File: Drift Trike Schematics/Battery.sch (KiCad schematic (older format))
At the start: 121 parts

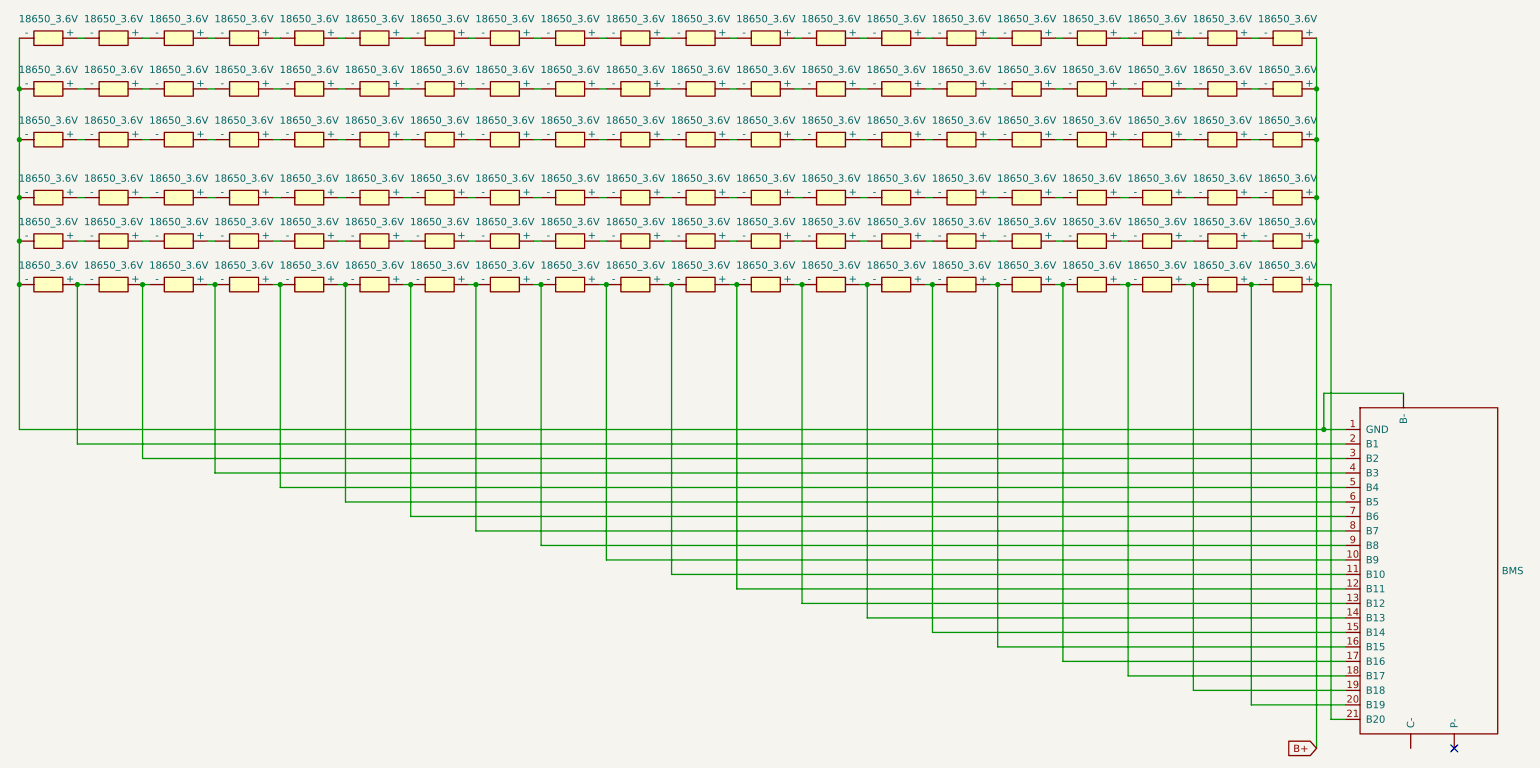
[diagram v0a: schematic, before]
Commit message: Small Fix
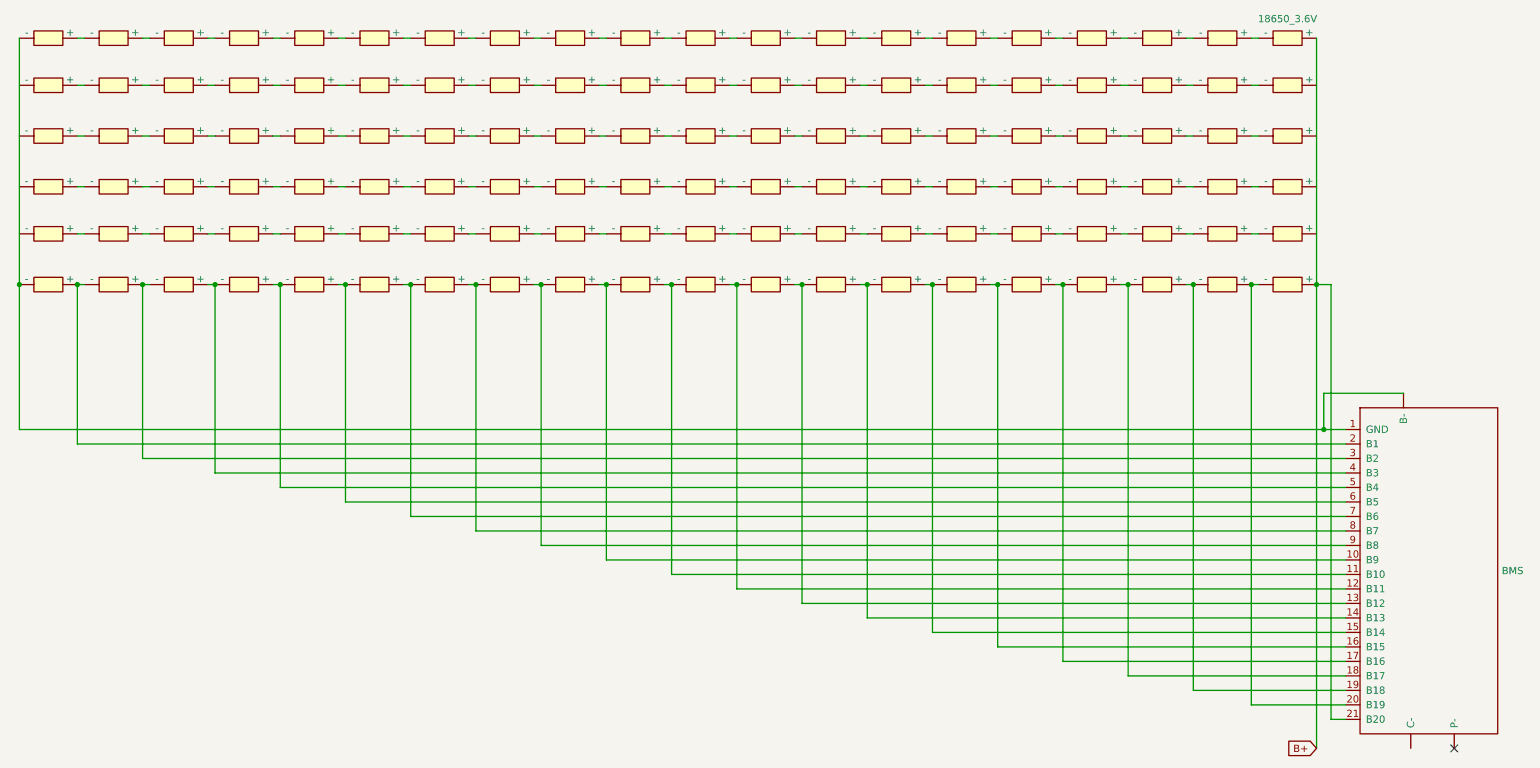
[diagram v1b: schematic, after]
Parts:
- removed U? (x80): 18650_3.6V, symbol trike_lib:18650_3.6V
- added U? (x80): 18650_3.6V, symbol trike_lib:18650_3.6V
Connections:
- new net: U?.1 (GND), U?.~ (-), U?.~ (-), U?.~ (P-)
- new net: U?.10 (B9), U?.~ (-), U?.~ (-)
- new net: U?.~ (-), U?.~ (-) (x76)
- now unconnected: U?.~ (P-)
